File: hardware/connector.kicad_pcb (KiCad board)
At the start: 4 copper layers, 20 x 22 mm, 2 parts, among them J1 AXK5F20347YG, J2 AXK5F20347YG

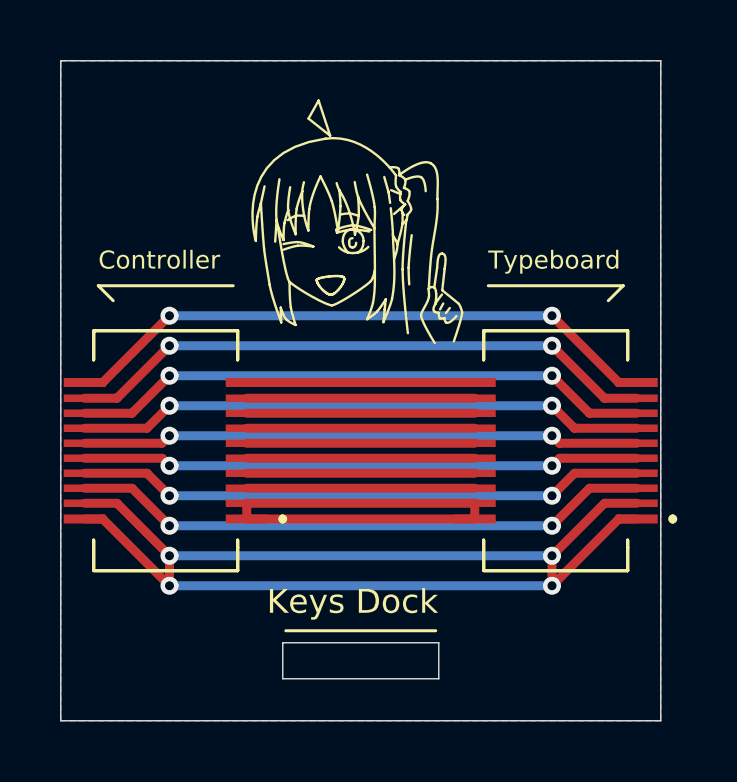
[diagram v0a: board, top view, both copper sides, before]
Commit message: :bug: improve hardware design
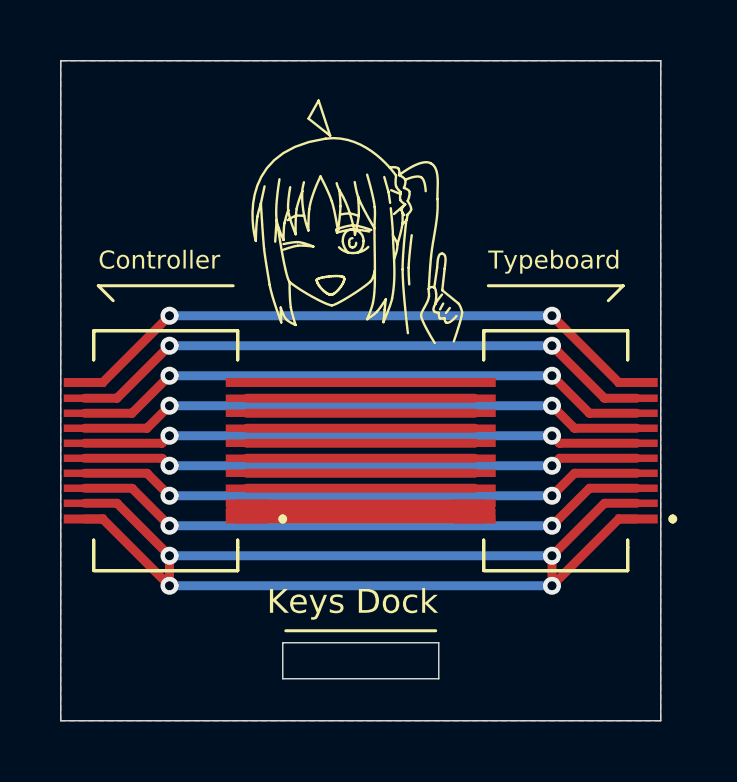
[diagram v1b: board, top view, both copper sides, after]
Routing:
- net P,+3.3: track 16.3 -> 8.21 mm
